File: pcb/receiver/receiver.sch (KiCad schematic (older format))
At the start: 35 parts, among them J101 Conn_01x02, Q101 BSS215PH6327XTSA1, Q102 MMBT2222A-7-F, U101 TPS63700DRCR, U102 NCP1403SNT1G

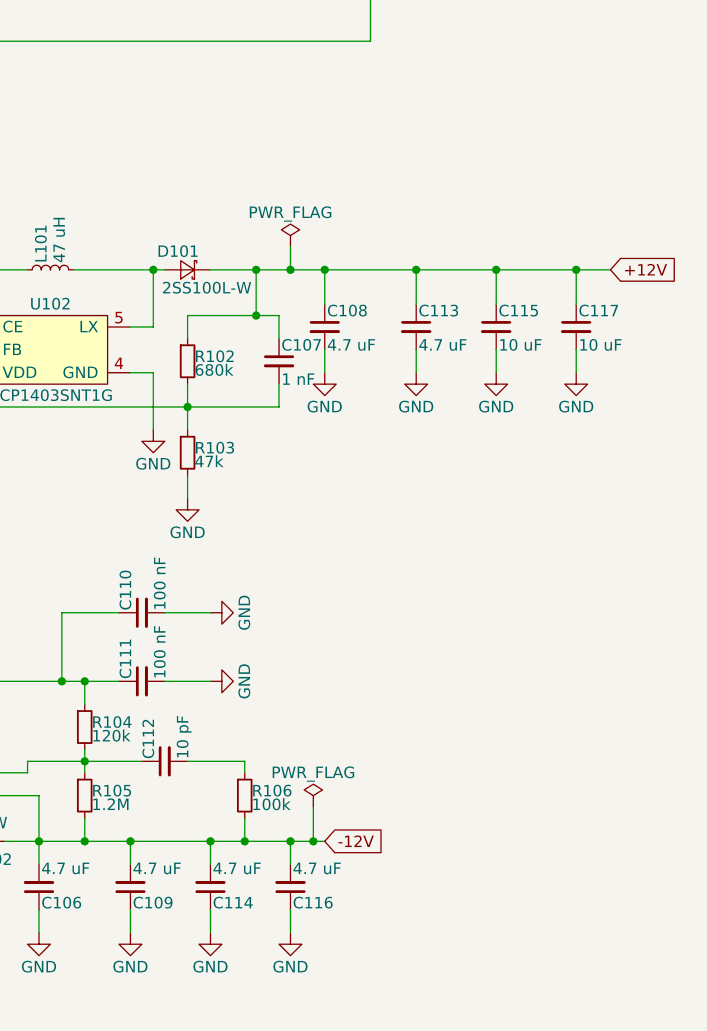
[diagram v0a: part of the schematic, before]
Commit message: Add copper fills and outline, autofill test point footprints, TODO finish placing test points and moving silkscreen
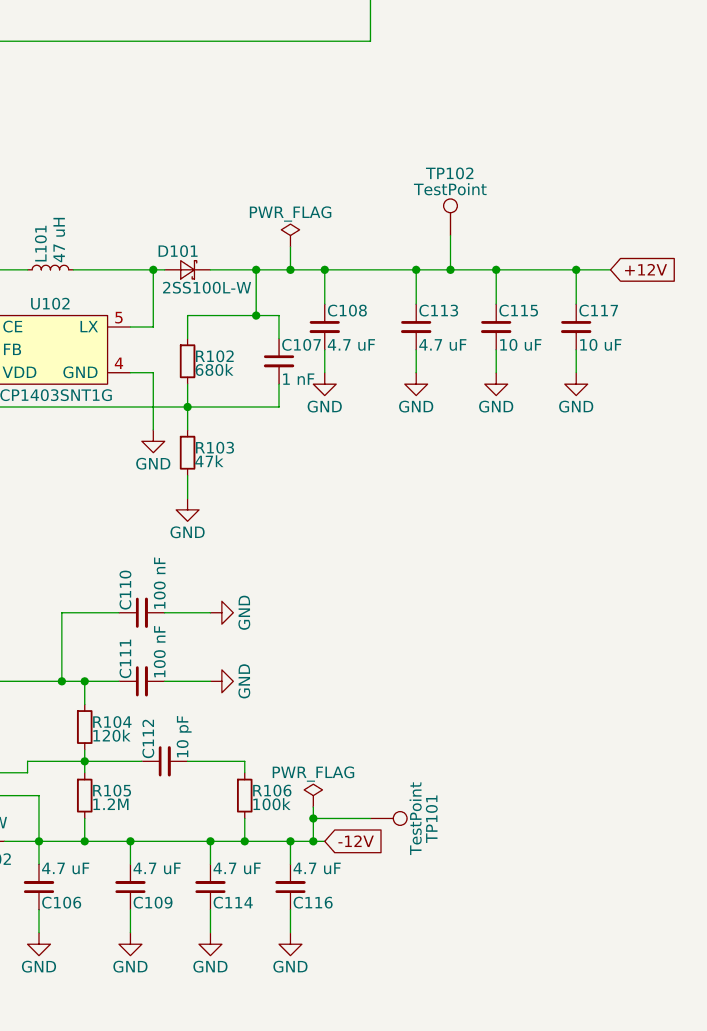
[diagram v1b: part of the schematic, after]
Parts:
- added TP101, TP102: TestPoint, Measurement_Points:Measurement_Point_Round-SMD-Pad_Small, symbol Connector:TestPoint
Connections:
- net +12V: now also TP102.1
- net -12V: now also TP101.1
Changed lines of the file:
@@
 Connection ~ 5750 4300
 Wire Wire Line
-	5750 4300 5400 4300
+	5750 4300 5550 4300
 Wire Wire Line
 	6100 4300 6100 4450
@@
 $EndComp
 Wire Wire Line
-	4950 6650 4950 6800
+	4950 6650 4950 6700
 Connection ~ 4950 6800
 Wire Wire Line
@@
 Wire Wire Line
 	1850 4550 2100 4550
+$Comp
+L Connector:TestPoint TP102
+U 1 1 5C2F2529
+P 5550 4150
+F 0 "TP102" H 5550 4420 50  0000 C CNN
+F 1 "TestPoint" H 5550 4350 50  0000 C CNN
+F 2 "Measurement_Points:Measurement_Point_Round-SMD-Pad_Small" H 5750 4150 50  0001 C CNN
+F 3 "~" H 5750 4150 50  0001 C CNN
+F 4 "NoPart" H 5750 4150 50  0001 C CNN "Mouser"
+	1    5550 4150
+	1    0    0    -1
+$EndComp
+Wire Wire Line
+	5550 4150 5550 4300
+Connection ~ 5550 4300
+Wire Wire Line
+	5550 4300 5400 4300
+$Comp
+L Connector:TestPoint TP101
+U 1 1 5C2F7F38
+P 5200 6700
+F 0 "TP101" H 5200 6970 50  0000 C CNN
+F 1 "TestPoint" H 5200 6900 50  0000 C CNN
+F 2 "Measurement_Points:Measurement_Point_Round-SMD-Pad_Small" H 5400 6700 50  0001 C CNN
+F 3 "~" H 5400 6700 50  0001 C CNN
+F 4 "NoPart" H 5200 6700 50  0001 C CNN "Mouser"
+	1    5200 6700
+	0    1    1    0
+$EndComp
+Wire Wire Line
+	5200 6700 4950 6700
+Connection ~ 4950 6700
+Wire Wire Line
+	4950 6700 4950 6800
 $EndSCHEMATC
